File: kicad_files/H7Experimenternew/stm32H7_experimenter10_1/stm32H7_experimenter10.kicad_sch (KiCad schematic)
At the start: 77 parts, among them IC1 AD8659, IC2 78TV, IC3 AD8659, IC5 6N138, P1 RK09SONGHUEI, P2 RK09SONGHUEI, P3 RK09SONGHUEI, P4 RK09SONGHUEI, P5 RK09SONGHUEI, P6 RK09SONGHUEI

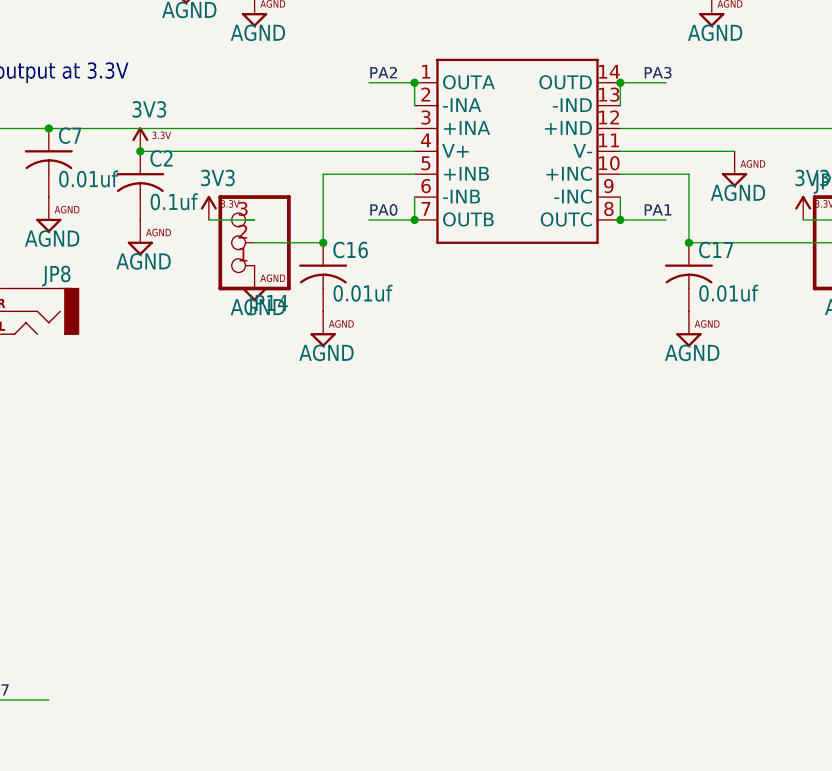
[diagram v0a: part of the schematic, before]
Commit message: experimenter kicad
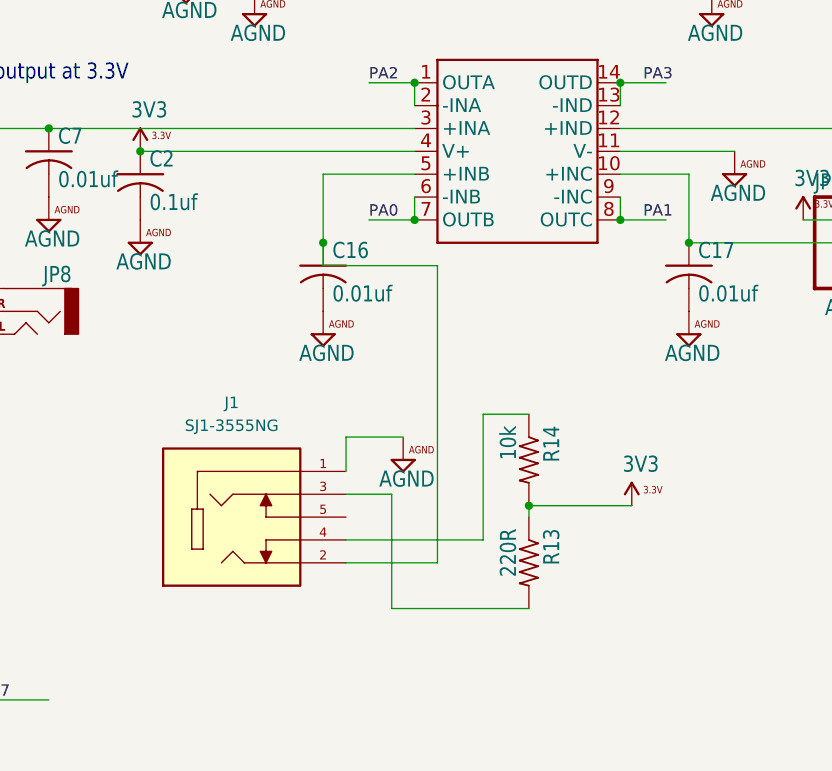
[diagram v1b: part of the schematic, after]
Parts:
- removed JP14: PINHD-1X3, stm32H7_experimenter10:1X03, symbol stm32H7_experimenter10-eagle-import:PINHD-1X3
- added J1: SJ1-3555NG, Snapeda:CUI_SJ1-3555NG, symbol Snapeda:SJ1-3555NG
- added R13: 220R, stm32H7_experimenter10:0204_5, symbol stm32H7_experimenter10-eagle-import:R-US_0204/5
- added R14: 10k, stm32H7_experimenter10:0204_5, symbol stm32H7_experimenter10-eagle-import:R-US_0204/5
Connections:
- net 3V3: now also R13.1, R14.2
- net AGND: now also J1.1
- net at C16.1, IC3.5 (+INB): now also J1.2
- new net: J1.4, R14.1
- new net: J1.3, R13.2
